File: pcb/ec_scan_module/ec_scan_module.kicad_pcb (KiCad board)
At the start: 2 copper layers, 21.3 x 24 mm, 17 parts, among them J2 Conn_01x08, J3 Conn_01x08, U2 TLV9061IDBVR, U3 74HC4051

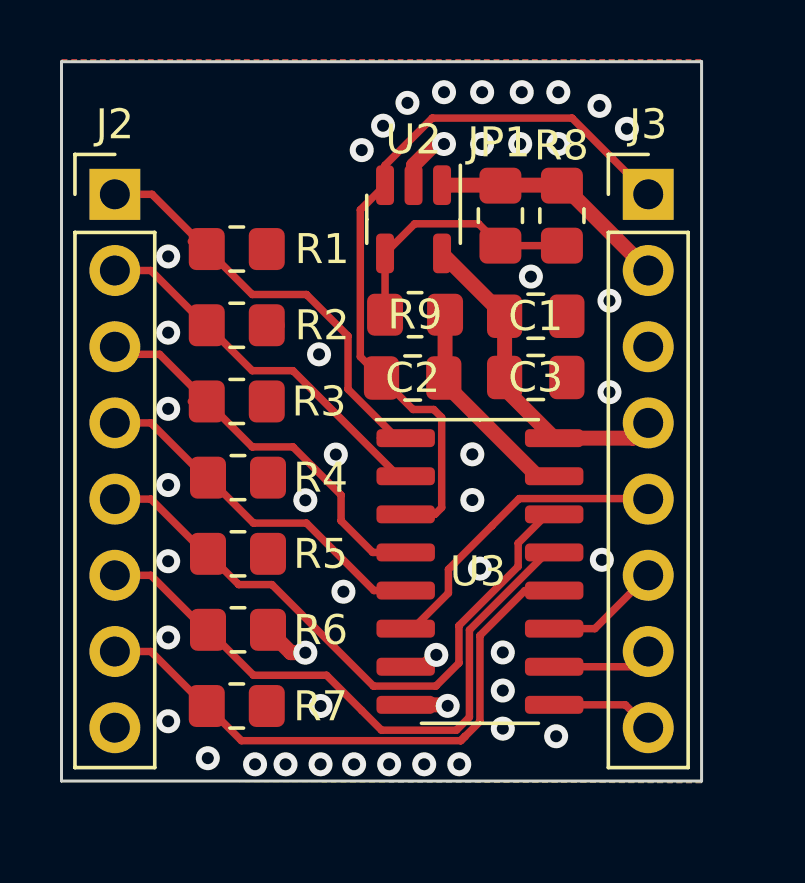
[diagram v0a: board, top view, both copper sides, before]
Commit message: modify
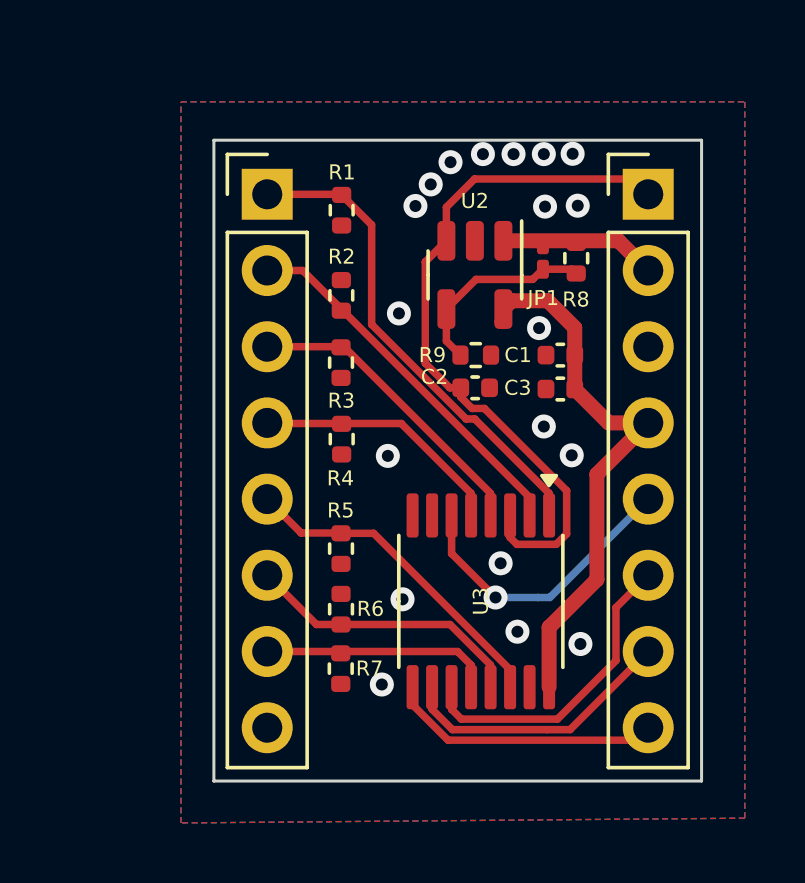
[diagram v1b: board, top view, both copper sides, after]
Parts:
- C1, C2, C3: footprint Capacitor_SMD:C_0805_2012Metric_Pad1.18x1.45mm_HandSolder -> Capacitor_SMD:C_0402_1005Metric
- JP1: footprint Resistor_SMD:R_0805_2012Metric_Pad1.20x1.40mm_HandSolder -> Resistor_SMD:R_0201_0603Metric_Pad0.64x0.40mm_HandSolder
- R1, R2, R3, R4, R5, R6, R7, R8, R9: footprint Resistor_SMD:R_0805_2012Metric_Pad1.20x1.40mm_HandSolder -> Resistor_SMD:R_0402_1005Metric
- U3: footprint Package_SO:SOIC-16_3.9x9.9mm_P1.27mm -> Package_SO:TSSOP-16_4.4x5mm_P0.65mm
- moved J2 5.08 mm to (83.9, 72.4)
- moved R1 3.73 mm to (86.3, 72.9), turned to -90 degrees
- moved R3 3.71 mm to (86.3, 78.0), turned to -90 degrees
- moved R4 3.69 mm to (86.3, 80.5), turned to -90 degrees
- moved R7 3.68 mm to (86.3, 88.2), turned to -90 degrees
- moved R2 3.63 mm to (86.3, 75.8), turned to 90 degrees
- moved R6 3.50 mm to (86.3, 86.2), turned to 90 degrees
- moved R5 3.44 mm to (86.3, 84.2), turned to -90 degrees
- moved U2 2.76 mm to (90.8, 75.1)
- moved R9 2.43 mm to (90.8, 77.7)
- moved C2 2.11 mm to (90.8, 78.8)
- moved JP1 1.98 mm to (93.1, 74.5)
- moved C1 1.53 mm to (93.6, 77.7), turned to 180 degrees
- moved R8 1.50 mm to (94.2, 74.5)
- moved U3 0.99 mm to (91.0, 86.0), turned to -90 degrees
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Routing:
- net GND: track 14.7 -> 0.00 mm, vias 47 -> 19
- net COL6: track 20.1 -> 7.72 mm
- net COL5: track 21.3 -> 9.42 mm
- net COL4: track 21.5 -> 11.5 mm
- net POWER: track 11.3 -> 18.1 mm
- net SEL0: track 3.87 -> 10.4 mm
- net SEL1: track 3.35 -> 9.85 mm
- net SEL2: track 3.75 -> 9.10 mm
- net COL3: track 12.3 -> 8.59 mm
- net COL2: track 13.8 -> 10.2 mm
- net ADC: track 8.35 -> 5.24 mm
- net Net-(JP1-B): track 8.65 -> 6.67 mm
- net DISCHARGE: track 25.0 -> 23.8 mm
- net COL1: track 13.6 -> 12.5 mm
- net EN: track 10.4 -> 9.79 mm, vias 0 -> 1
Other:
- board size 21.3 x 24 mm -> 16.3 x 21.4 mm
